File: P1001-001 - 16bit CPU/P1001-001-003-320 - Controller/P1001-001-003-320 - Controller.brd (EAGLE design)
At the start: 200 x 152 mm, 129 parts, among them IC10 74ALS00D, IC21 74LS138D, IC22 74LS138D, IC27 MEGA8535-A, IC3 74LS138D, IC4 74LS138D, IC5 74LS138D, J1 22-27-2041-04

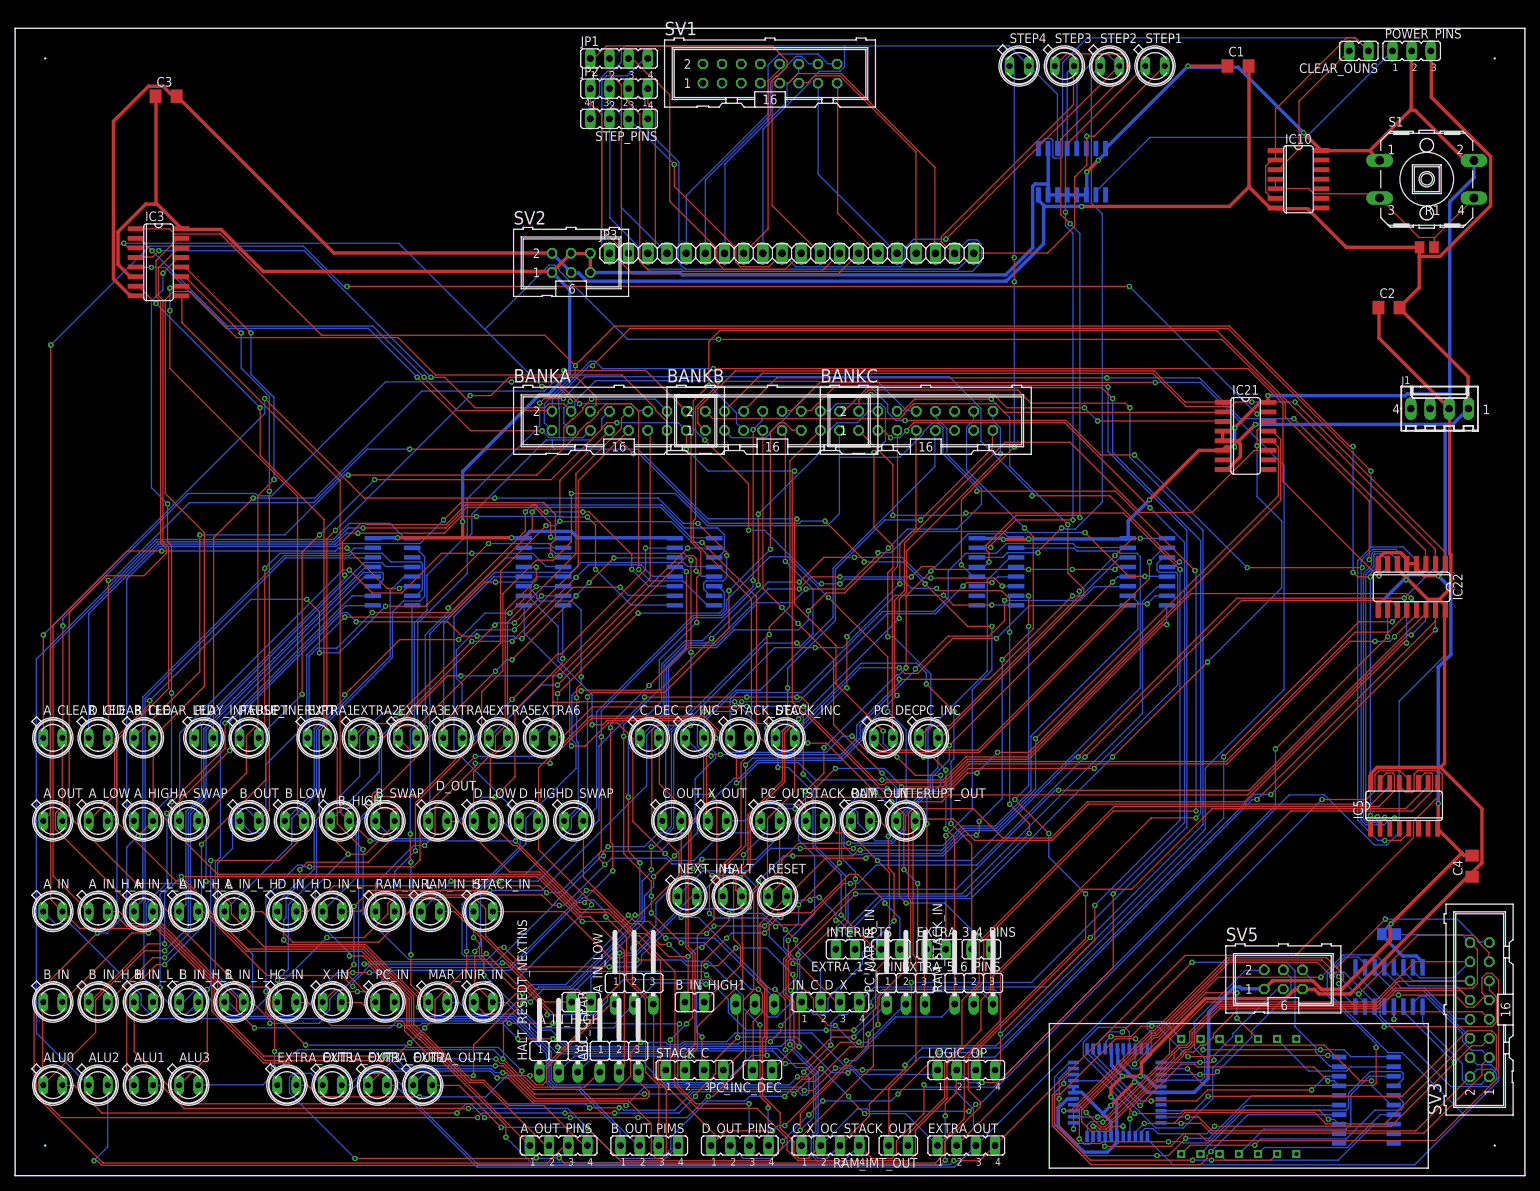
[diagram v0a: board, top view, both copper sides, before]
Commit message: Check in the first try at soldering up the board
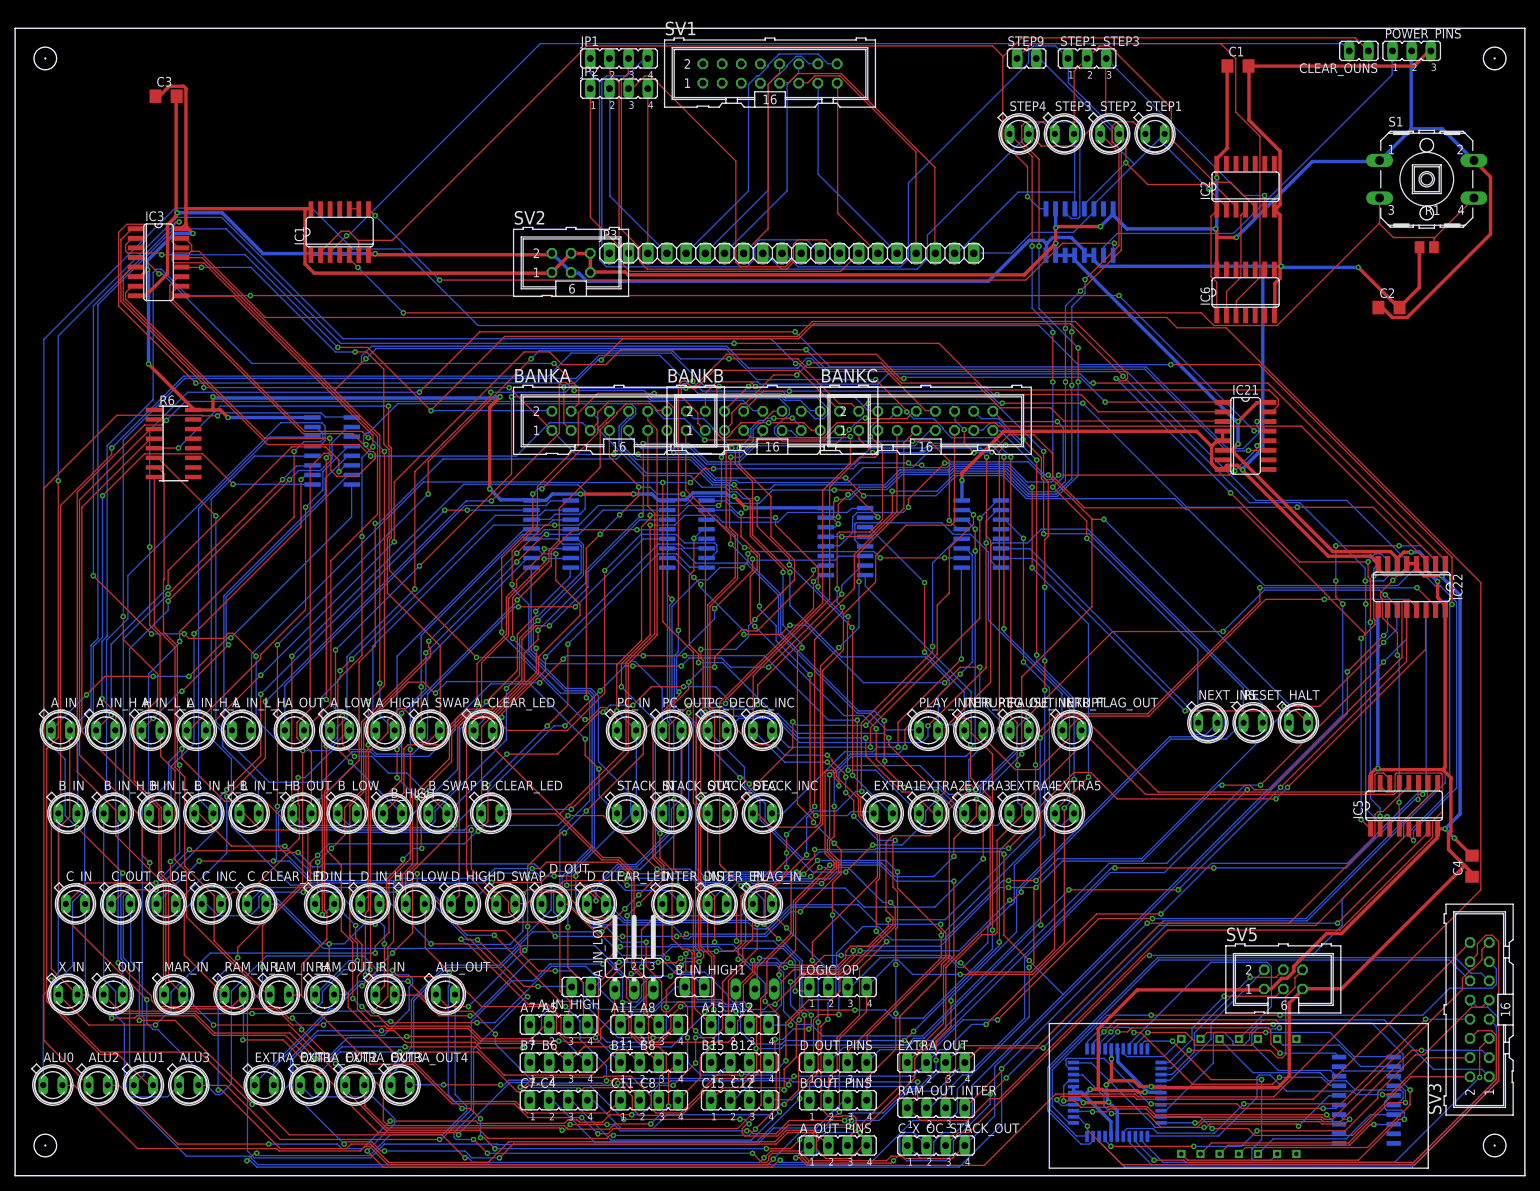
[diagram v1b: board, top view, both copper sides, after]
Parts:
- removed ABC_CLEAR, HALT_RESEDT_NEXTINS, PC_MAR_IR_IN, RAM_STACK_IN: (no value), jumper:JP2W
- removed B_OUT_PIMS, IN_C_D_X, STACK_C, STEP_PINS: (no value), jumper:JP4
- removed EXTRA6, INTERUPT_OUT: (no value), led:SFH482
- removed EXTRA_1_2_PINS, EXTRA_3_4_PINS, EXTRA_5_6_PINS, INTERUPTS, PC_INC_DEC, RAM_IMT_OUT: (no value), jumper:JP1
- removed IC10: 74ALS00D, 74xx-us:SO14
- removed J1: 22-27-2041-04, con-molex:6410-04
- removed PULL_DOWN: (no value), rcl:M0805
- removed R10: (no value), resistor-bourns:SO16
- added A11_A8, A15_A12, A7_A5, B11_B8, B15_B12, B7_B6, B_OUT_PINS, C11_C8, C15_C12, C7-C4, RAM_OUT_INTER: (no value), jumper:JP4
- added ALU_OUT, C_CLEAR_LED, FLAG_IN, INTER_DIS, INTER_EN, INTR_FLAG_OUT, INTR_REG_OUT: (no value), led:SFH482
- added IC1: 74ALS00D, 74xx-us:SO14
- added IC2: 74ALS02D, 74xx-us:SO14
- added IC6: 74ALS08D, 74xx-us:SO14
- added R6: (no value), resistor-bourns:SO16
- added STEP1_STEP3: (no value), jumper:JP2
- added STEP9: (no value), jumper:JP1
- moved PAUSE_INERUPT 102.0 mm to (133.0, 59.0)
- moved PLAY_INTERUPT 96.0 mm to (121.0, 59.0)
- moved X_OUT 83.2 mm to (13.0, 24.0)
- moved HALT 78.4 mm to (170.0, 60.0)
- moved EXTRA1 75.7 mm to (115.0, 48.0)
- moved EXTRA2 75.7 mm to (121.0, 48.0)
- moved EXTRA3 75.7 mm to (127.0, 48.0)
- moved EXTRA4 75.7 mm to (133.0, 48.0)
- moved EXTRA5 75.7 mm to (139.0, 48.0)
- moved RAM_OUT 74.6 mm to (41.0, 24.0)
- moved C_OUT 73.8 mm to (14.0, 36.0)
- moved NEXT_INS 72.7 mm to (158.0, 60.0)
- moved D_CLEAR_LED 69.6 mm to (77.0, 36.0)
- moved C_DEC 67.7 mm to (20.0, 36.0)
- moved C_INC 67.7 mm to (26.0, 36.0)
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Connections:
- new net FIRST_STEP: IC6.3, STEP9.1
- new net N$42: EXTRA5.K, R5.3
- new net N$50: EXTRA_OUT.3, EXTRA_OUT3.K, IC5.9
- new net N$56: EXTRA_OUT.4, EXTRA_OUT4.K, IC5.7
- new net N$57: EXTRA_OUT3.A, R2.9
- new net N$58: EXTRA_OUT4.A, R2.10
- new net N$59: R5.8, RESET.K
- new net N$60: HALT.K, R5.7
- new net N$61: IC2.4, IC6.2
- new net N$62: IC2.1, IC6.1
- new net N$63: NEXT_INS.K, R5.6
- net !CLEAR: now also IC1.1, IC1.2, IC1.6; no longer IC10.1, IC10.2, IC10.6
- net CLEAR: now also IC1.3; no longer IC10.3
- net DATAA10: now also A11_A8.3, A_CLEAR_LED.K; no longer EXTRA6.K, EXTRA_5_6_PINS.2
- net DATAA11: now also A11_A8.4, B_CLEAR_LED.K; no longer ABC_CLEAR.1, A_CLEAR_LED.K
- net DATAA12: now also A15_A12.1, C_CLEAR_LED.K; no longer ABC_CLEAR.2, B_CLEAR_LED.K
- net DATAA13: now also A15_A12.2; no longer ABC_CLEAR.3
- net DATAA14: now also A15_A12.3; no longer INTERUPTS.1
- net DATAA15: now also A15_A12.4; no longer INTERUPTS.2
- net DATAA5: now also A7_A5.2; no longer EXTRA_1_2_PINS.1
- net DATAA6: now also A7_A5.3; no longer EXTRA_1_2_PINS.2
- net DATAA7: now also A7_A5.4; no longer EXTRA_3_4_PINS.1
- net DATAA8: now also A11_A8.1; no longer EXTRA_3_4_PINS.2
- net DATAA9: now also A11_A8.2, EXTRA5.A; no longer EXTRA5.K, EXTRA_5_6_PINS.1
- net DATAB10: now also B11_B8.3; no longer PC_MAR_IR_IN.1
- net DATAB11: now also B11_B8.4; no longer PC_MAR_IR_IN.2
- net DATAB12: now also B15_B12.1; no longer PC_MAR_IR_IN.3
- net DATAB13: now also B15_B12.2; no longer RAM_STACK_IN.1
- net DATAB14: now also B15_B12.3; no longer RAM_STACK_IN.2
- net DATAB15: now also B15_B12.4; no longer RAM_STACK_IN.3
- net DATAB4: no longer PC_INC_DEC.2
- net DATAB6: now also B7_B6.3; no longer IN_C_D_X.1
- net DATAB7: now also B7_B6.4; no longer IN_C_D_X.2
- net DATAB8: now also B11_B8.1; no longer IN_C_D_X.3
- net DATAB9: now also B11_B8.2; no longer IN_C_D_X.4
- net DATAC10: now also C11_C8.3, FLAG_IN.A
- net DATAC11: now also C11_C8.4, INTER_EN.A
- net DATAC12: now also C15_C12.1, INTER_DIS.A
- net DATAC13: now also C15_C12.2, RESET.A; no longer HALT_RESEDT_NEXTINS.3, RESET.K
- net DATAC14: now also C15_C12.3, HALT.A; no longer HALT.K, HALT_RESEDT_NEXTINS.2
- net DATAC15: now also C15_C12.4, NEXT_INS.A; no longer HALT_RESEDT_NEXTINS.1, NEXT_INS.K
- net DATAC4: now also C7-C4.1, PC_DEC.A; no longer PC_DEC.K
- net DATAC5: now also C7-C4.2, PC_INC.A; no longer PC_INC.K, PC_INC_DEC.1
- net DATAC6: now also C7-C4.3, STACK_INC.A; no longer STACK_C.4, STACK_INC.K
- net DATAC7: now also C7-C4.4, STACK_DEC.A; no longer STACK_C.3, STACK_DEC.K
- net DATAC8: now also C11_C8.1, C_INC.A; no longer C_INC.K, STACK_C.2
- net DATAC9: now also C11_C8.2, C_DEC.A; no longer C_DEC.K, STACK_C.1
- net EXTERN_BUS0: no longer R10.1
- net EXTERN_BUS1: no longer R10.9
- net EXTERN_BUS10: no longer R10.6
- net EXTERN_BUS11: no longer R10.14
- net EXTERN_BUS12: no longer R10.7
- net EXTERN_BUS13: no longer R10.15
- net EXTERN_BUS14: no longer R10.8
- net EXTERN_BUS15: no longer PULL_DOWN.1
- net EXTERN_BUS2: no longer R10.2
- net EXTERN_BUS3: no longer R10.10
- net EXTERN_BUS4: no longer R10.3
- net EXTERN_BUS5: no longer R10.11
- net EXTERN_BUS6: no longer R10.4
- net EXTERN_BUS7: no longer R10.12
- net EXTERN_BUS8: no longer R10.5
- net EXTERN_BUS9: no longer R10.13
- net GND: now also IC1.7, IC2.7, IC6.7, R5.16, U$4.3, U$4.4; no longer IC10.7, J1.1, PULL_DOWN.2, R10.16
- net IN_BUS0: now also IC2.2, STEP9.2; no longer STEP_PINS.1
- net IN_BUS1: now also IC2.3, STEP1_STEP3.1; no longer STEP_PINS.2
- net IN_BUS2: now also IC2.5, STEP1_STEP3.2; no longer STEP_PINS.3
- net IN_BUS3: now also IC2.6, STEP1_STEP3.3; no longer STEP_PINS.4
- net N$1: now also IC1.4, IC1.5; no longer IC10.4, IC10.5
- net N$106: now also RAM_OUT_INTER.1; no longer RAM_IMT_OUT.1
- net N$107: now also INTR_REG_OUT.K, RAM_OUT_INTER.2; no longer INTERUPT_OUT.K, RAM_IMT_OUT.2
- net N$108: now also INTR_FLAG_OUT.K, RAM_OUT_INTER.3; no longer EXTRA_OUT.4, EXTRA_OUT1.K
- net N$109: now also ALU_OUT.K, RAM_OUT_INTER.4; no longer EXTRA_OUT.3, EXTRA_OUT2.K
- net N$110: now also EXTRA_OUT.1, EXTRA_OUT1.K; no longer EXTRA_OUT.2, EXTRA_OUT3.K
- net N$111: now also EXTRA_OUT.2, EXTRA_OUT2.K; no longer EXTRA_OUT.1, EXTRA_OUT4.K
- net N$113: now also EXTRA_OUT2.A; no longer EXTRA_OUT4.A
- net N$114: now also EXTRA_OUT1.A; no longer EXTRA_OUT3.A
- net N$115: now also ALU_OUT.A; no longer EXTRA_OUT2.A
- net N$116: now also INTR_FLAG_OUT.A; no longer EXTRA_OUT1.A
- net N$118: now also INTR_REG_OUT.A; no longer INTERUPT_OUT.A
- net N$16: now also PC_INC.K; no longer PC_INC.A
- net N$17: now also PC_DEC.K; no longer PC_DEC.A
- net N$18: now also R6.8, RAM_IN_H.A; no longer IR_IN.A, R5.3
- net N$19: now also R6.7, RAM_IN_L.A; no longer MAR_IN.A, R5.4
- net N$20: now also R6.6, STACK_IN.A; no longer PC_IN.A, R5.5
- net N$21: now also PC_IN.A, R6.5; no longer R5.6, STACK_IN.A
- net N$22: now also MAR_IN.A, R6.4; no longer R5.7, RAM_IN_L.A
- net N$23: now also IR_IN.A, R6.3; no longer R5.8, RAM_IN_H.A
- net N$24: now also INTER_DIS.K; no longer NEXT_INS.A
- net N$25: now also STACK_DEC.K; no longer STACK_DEC.A
- net N$26: now also C_INC.K; no longer C_INC.A
- net N$27: now also C_DEC.K; no longer C_DEC.A
- net N$28: now also FLAG_IN.K; no longer RESET.A
- net N$29: now also INTER_EN.K; no longer HALT.A
- net N$30: now also STACK_INC.K; no longer STACK_INC.A
- net N$43: now also IC1.8, U$4.1; no longer EXTRA5.A, R8.5
- net N$7: now also A_CLEAR_LED.A; no longer EXTRA6.A
- net N$79: now also B_OUT_PINS.1; no longer B_OUT_PIMS.1
- net N$8: now also C_CLEAR_LED.A; no longer B_CLEAR_LED.A
- net N$80: now also B_OUT_PINS.2; no longer B_OUT_PIMS.2
- net N$81: now also B_OUT_PINS.3; no longer B_OUT_PIMS.3
- net N$82: now also B_OUT_PINS.4; no longer B_OUT_PIMS.4
- net N$9: now also B_CLEAR_LED.A; no longer A_CLEAR_LED.A
- net NEXT_INS: now also IC1.10, IC1.9; no longer U$4.1
- net VCC: now also IC1.14, IC2.14, IC6.14, R6.16; no longer IC10.14, J1.2, R5.16, U$4.3, U$4.4
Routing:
- net N$75: track 170.0 -> 424.6 mm, vias 0 -> 1
- net N$88: track 177.0 -> 426.9 mm
- net N$50: track 0.00 -> 168.1 mm, vias 0 -> 6
- net DATAC12: track 0.00 -> 158.5 mm, vias 0 -> 7
- net N$56: track 0.00 -> 157.6 mm, vias 0 -> 8
- net N$57: track 0.00 -> 148.6 mm, vias 0 -> 9
- net N$1: track 33.8 -> 167.7 mm, vias 0 -> 2
- net DATAB4: track 231.4 -> 101.0 mm, vias 7 -> 0
- net CLEAR: track 20.0 -> 147.3 mm, vias 0 -> 1
- net DATAC4: track 41.1 -> 165.4 mm, vias 0 -> 5
- net DATAC11: track 0.00 -> 123.1 mm, vias 0 -> 8
- net DATAC10: track 0.00 -> 120.7 mm, vias 0 -> 3
- net N$19: track 188.5 -> 75.1 mm, vias 7 -> 2
- net N$58: track 0.00 -> 106.1 mm, vias 0 -> 7
- net DATAC8: track 101.1 -> 203.9 mm, vias 0 -> 7
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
